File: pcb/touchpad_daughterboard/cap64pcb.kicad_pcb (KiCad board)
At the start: 2 copper layers, 91.6 x 12 mm, 35 parts, among them J1 SM04B_SURS_TF, M1 Coin_Motor, Q1 BSS138, Q2 BSS138, U1 MPR121QR2, U2 SPX3819-3.3

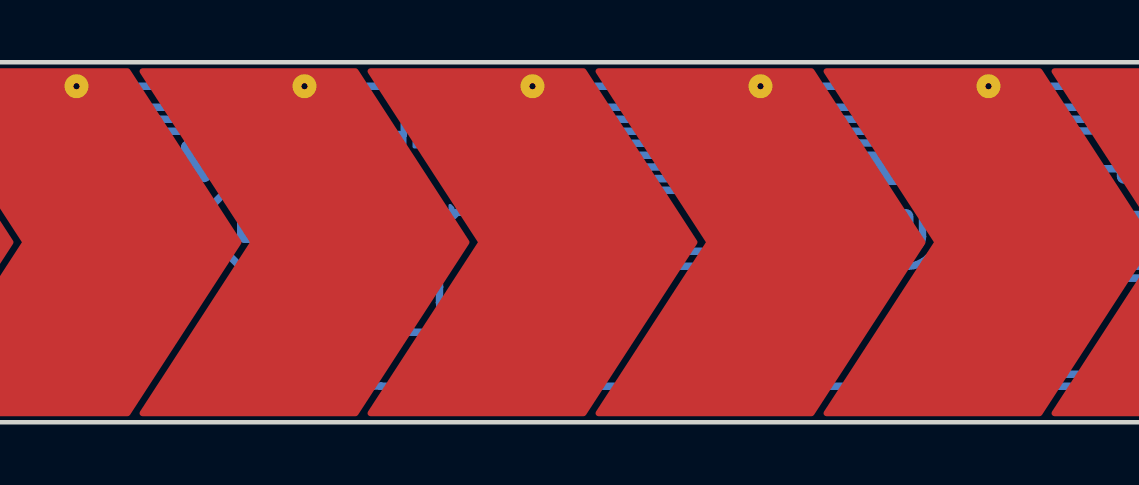
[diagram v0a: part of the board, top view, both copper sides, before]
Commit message: silks
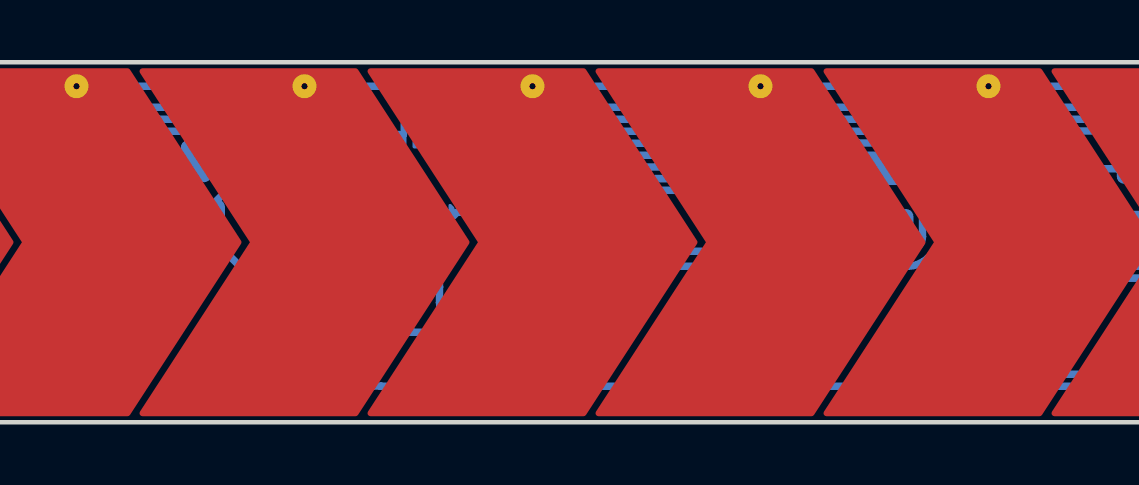
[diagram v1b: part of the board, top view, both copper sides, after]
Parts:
- moved C5 0.50 mm to (66.4, 44.3)
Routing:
- net Net-(C5-Pad1): track 5.10 -> 4.60 mm
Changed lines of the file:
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@@
       (effects (font (size 1 1) (thickness 0.15)) (justify mirror))
     )
-    (fp_text value "b" (at 0 -1.8) (layer "B.SilkS")
+    (fp_text value "b" (at 0 -1.7) (layer "B.SilkS")
       (effects (font (size 1.2 1.2) (thickness 0.3)) (justify mirror))
     )
@@
   )
   (footprint "Capacitor_SMD:C_0805_2012Metric" (layer "B.Cu")
-    (at 65.9 44.3 180)
+    (at 66.4 44.3 180)
     (descr "Capacitor SMD 0805 (2012 Metric), square (rectangular) end terminal, IPC_7351 nominal, (Body size source: IPC-SM-782 page 76, https://www.pcb-3d.com/wordpress/wp-content/uploads/ipc-sm-782a_amendment_1_and_2.pdf, https://docs.google.com/spreadsheets/d/1BsfQQcO9C6DZCsRaXUlFlo91Tg2WpOkGARC1WS5S8t0/edit?usp=sharing), generated with kicad-footprint-generator")
     (tags "capacitor")
@@
       (effects (font (size 1 1) (thickness 0.15)) (justify mirror))
     )
-    (fp_text value "MPR121QR2" (at 2.8 -1.05) (layer "B.SilkS")
+    (fp_text value "MPR121QR2" (at 2.8 -1.2) (layer "B.SilkS")
       (effects (font (size 1.2 1.2) (thickness 0.3)) (justify mirror))
     )
@@
       (effects (font (size 1 1) (thickness 0.15)) (justify mirror))
     )
-    (fp_text user "c" (at 1.1 1.8 180) (layer "B.SilkS")
+    (fp_text user "c" (at 1.1 1.7 180) (layer "B.SilkS")
       (effects (font (size 1.2 1.2) (thickness 0.3)) (justify mirror))
     )
@@
       (effects (font (size 1 1) (thickness 0.15)) (justify mirror))
     )
-    (fp_text user "a" (at -1.1 1.8 180) (layer "B.SilkS")
+    (fp_text user "a" (at -1.1 1.7 180) (layer "B.SilkS")
       (effects (font (size 1.2 1.2) (thickness 0.3)) (justify mirror))
     )
@@
       (effects (font (size 1 1) (thickness 0.15)) (justify mirror))
     )
-    (fp_text value "d" (at 0 -1.8) (layer "B.SilkS")
+    (fp_text value "d" (at 0 -1.7) (layer "B.SilkS")
       (effects (font (size 1.2 1.2) (thickness 0.3)) (justify mirror))
     )
@@
       (effects (font (size 1 1) (thickness 0.15)) (justify mirror))
     )
-    (fp_text value "INT" (at -2.4 0.3 -180) (layer "B.SilkS")
-      (effects (font (size 1.2 1.2) (thickness 0.3)) (justify mirror))
+    (fp_text value "INT" (at -2.4 0.5 -180) (layer "B.SilkS")
+      (effects (font (size 1.2 1.2) (thickness 0.3) italic) (justify mirror))
     )
     (fp_text user "${REFERENCE}" (at 0 0 90) (layer "B.Fab")
@@
   (gr_line (start 36.3 39) (end 123.7 39) (layer "Edge.Cuts") (width 0.15))
   (gr_line (start 125.8 48.9) (end 125.8 41.1) (layer "Edge.Cuts") (width 0.15))
-  (gr_text "0x5[abcd]" (at 61.8 46.5) (layer "B.SilkS")
-    (effects (font (size 1.2 1.2) (thickness 0.3)) (justify mirror))
+  (gr_text "0x5[abcd]" (at 71 49.9) (layer "B.SilkS")
+    (effects (font (size 1 1) (thickness 0.2)) (justify mirror))
   )
   (gr_text "gnd" (at 111.9 45.3 90) (layer "B.SilkS")
@@
     (effects (font (size 1 1) (thickness 0.2)) (justify left mirror))
   )
+  (gr_text "cap" (at 52.8 43.7) (layer "B.SilkS")
+    (effects (font (size 1.5 1.5) (thickness 0.3)) (justify mirror))
+  )
   (gr_text "sda" (at 108 45.2 90) (layer "B.SilkS")
     (effects (font (size 1 1) (thickness 0.2)) (justify left mirror))
   )
-  (gr_text "biddle" (at 46.7 44.3) (layer "B.SilkS")
+  (gr_text "biddle" (at 47.3 45.999999) (layer "B.SilkS")
     (effects (font (size 1.5 1.5) (thickness 0.3)) (justify mirror))
   )
@@
     (effects (font (size 1.2 1.2) (thickness 0.3)) (justify left mirror))
   )
+  (gr_text "beady" (at 54.1 45.999999) (layer "B.SilkS")
+    (effects (font (size 1.5 1.5) (thickness 0.3)) (justify mirror))
+  )
   (gr_text "vib" (at 109.3 45.3 90) (layer "B.SilkS")
     (effects (font (size 1 1) (thickness 0.2)) (justify left mirror))
@@
     (effects (font (size 1.2 1.2) (thickness 0.3)) (justify mirror))
   )
-  (gr_text "64" (at 48.7 42) (layer "B.SilkS")
-    (effects (font (size 1.5 1.5) (thickness 0.3)) (justify mirror))
-  )
-  (gr_text "cap" (at 52.2 42) (layer "B.Mask")
-    (effects (font (size 1.5 1.5) (thickness 0.3)) (justify mirror))
-  )
-  (gr_text "beady" (at 53.5 44.3) (layer "B.Mask")
+  (gr_text "64" (at 49.3 43.7) (layer "B.SilkS")
     (effects (font (size 1.5 1.5) (thickness 0.3)) (justify mirror))
   )
@@
   (segment (start 104.7 42.505723) (end 103.15 44.055723) (width 0.25) (layer "B.Cu") (net 1))
   (segment (start 104.7 44.055723) (end 104.05 44.705723) (width 0.25) (layer "B.Cu") (net 2))
+  (segment (start 67.15 46.5) (end 65.45 44.8) (width 0.25) (layer "B.Cu") (net 2))
   (segment (start 110.2 42.35) (end 110.2 41.27904) (width 0.25) (layer "B.Cu") (net 2))
   (segment (start 101.6 44.705723) (end 98.755723 44.705723) (width 0.25) (layer "B.Cu") (net 2))
   (segment (start 106.5 44.3) (end 104.944277 44.3) (width 0.25) (layer "B.Cu") (net 2))
-  (segment (start 64.9875 44.3) (end 65.9875 43.3) (width 0.25) (layer "B.Cu") (net 2))
-  (segment (start 67.5 46.979022) (end 69.735192 49.214214) (width 0.25) (layer "B.Cu") (net 2))
-  (segment (start 64.95 44.3) (end 64.9875 44.3) (width 0.25) (layer "B.Cu") (net 2))
+  (segment (start 67.5 46.979022) (end 67.5 46.5) (width 0.25) (layer "B.Cu") (net 2))
   (segment (start 98.5 44.45) (end 96.4 44.45) (width 0.25) (layer "B.Cu") (net 2))
   (segment (start 98.755723 44.705723) (end 98.5 44.45) (width 0.25) (layer "B.Cu") (net 2))
@@
   (segment (start 65.9875 43.3) (end 64.9875 42.3) (width 0.25) (layer "B.Cu") (net 2))
   (segment (start 110.2 41.27904) (end 107.72096 41.27904) (width 0.25) (layer "B.Cu") (net 2))
-  (segment (start 67.5 46.5) (end 67.15 46.5) (width 0.25) (layer "B.Cu") (net 2))
+  (segment (start 65.45 44.3) (end 65.45 43.8375) (width 0.25) (layer "B.Cu") (net 2))
+  (segment (start 65.45 43.8375) (end 65.9875 43.3) (width 0.25) (layer "B.Cu") (net 2))
   (segment (start 71.3125 43.6) (end 70.2 43.6) (width 0.25) (layer "B.Cu") (net 2))
   (segment (start 102.7375 43.105723) (end 101.6 43.105723) (width 0.25) (layer "B.Cu") (net 2))
+  (segment (start 69.735192 49.214214) (end 67.5 46.979022) (width 0.25) (layer "B.Cu") (net 2))
   (segment (start 110.2 43.3) (end 110.2 42.35) (width 0.25) (layer "B.Cu") (net 2))
   (segment (start 90.3 49.8) (end 108.3 49.8) (width 0.25) (layer "B.Cu") (net 2))
@@
   (segment (start 69.9 43.3) (end 65.9875 43.3) (width 0.25) (layer "B.Cu") (net 2))
   (segment (start 107.72096 41.27904) (end 106.5 42.5) (width 0.25) (layer "B.Cu") (net 2))
-  (segment (start 71.149405 49.8) (end 90.3 49.8) (width 0.25) (layer "B.Cu") (net 2))
-  (segment (start 67.5 46.5) (end 67.5 46.979022) (width 0.25) (layer "B.Cu") (net 2))
+  (segment (start 90.3 49.8) (end 71.149405 49.8) (width 0.25) (layer "B.Cu") (net 2))
   (segment (start 70.2 43.6) (end 69.9 43.3) (width 0.25) (layer "B.Cu") (net 2))
-  (segment (start 67.15 46.5) (end 64.95 44.3) (width 0.25) (layer "B.Cu") (net 2))
+  (segment (start 65.45 44.8) (end 65.45 44.3) (width 0.25) (layer "B.Cu") (net 2))
   (segment (start 112.297666 44.302334) (end 112.3 44.3) (width 0.25) (layer "B.Cu") (net 2))
+  (segment (start 67.5 46.5) (end 67.15 46.5) (width 0.25) (layer "B.Cu") (net 2))
   (segment (start 101.6 44.705723) (end 101.6 43.105723) (width 0.25) (layer "B.Cu") (net 2))
-  (arc (start 71.149405 49.8) (mid 70.384038 49.647759) (end 69.735192 49.214214) (width 0.25) (layer "B.Cu") (net 2))
   (arc (start 108.3 49.8) (mid 111.058162 48.696988) (end 112.297666 45.996393) (width 0.25) (layer "B.Cu") (net 2))
   (arc (start 111.2 44.3) (mid 110.492893 44.007107) (end 110.2 43.3) (width 0.25) (layer "B.Cu") (net 2))
+  (arc (start 71.149405 49.8) (mid 70.384038 49.647759) (end 69.735192 49.214214) (width 0.25) (layer "B.Cu") (net 2))
   (segment (start 98.5 42.55) (end 98.956777 42.55) (width 0.25) (layer "B.Cu") (net 3))
   (segment (start 98.956777 42.55) (end 100.4625 44.055723) (width 0.25) (layer "B.Cu") (net 3))
@@
   (arc (start 103.682843 47.923935) (mid 103.769552 47.794166) (end 103.8 47.641093) (width 0.25) (layer "B.Cu") (net 4))
   (arc (start 103.8 47.521181) (mid 103.830448 47.368107) (end 103.917158 47.238338) (width 0.25) (layer "B.Cu") (net 4))
-  (segment (start 66.9625 44.1875) (end 66.85 44.3) (width 0.25) (layer "B.Cu") (net 5))
-  (segment (start 71.9 44.1875) (end 66.9625 44.1875) (width 0.25) (layer "B.Cu") (net 5))
+  (segment (start 71.9 44.1875) (end 67.4625 44.1875) (width 0.25) (layer "B.Cu") (net 5))
+  (segment (start 67.4625 44.1875) (end 67.35 44.3) (width 0.25) (layer "B.Cu") (net 5))
   (segment (start 105.4 49.4) (end 93.728427 49.4) (width 0.25) (layer "B.Cu") (net 6))
   (segment (start 92.314213 48.814213) (end 90.3 46.8) (width 0.25) (layer "B.Cu") (net 6))
